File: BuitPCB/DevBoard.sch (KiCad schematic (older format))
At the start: 1 part, among them U1 Teensy4.1

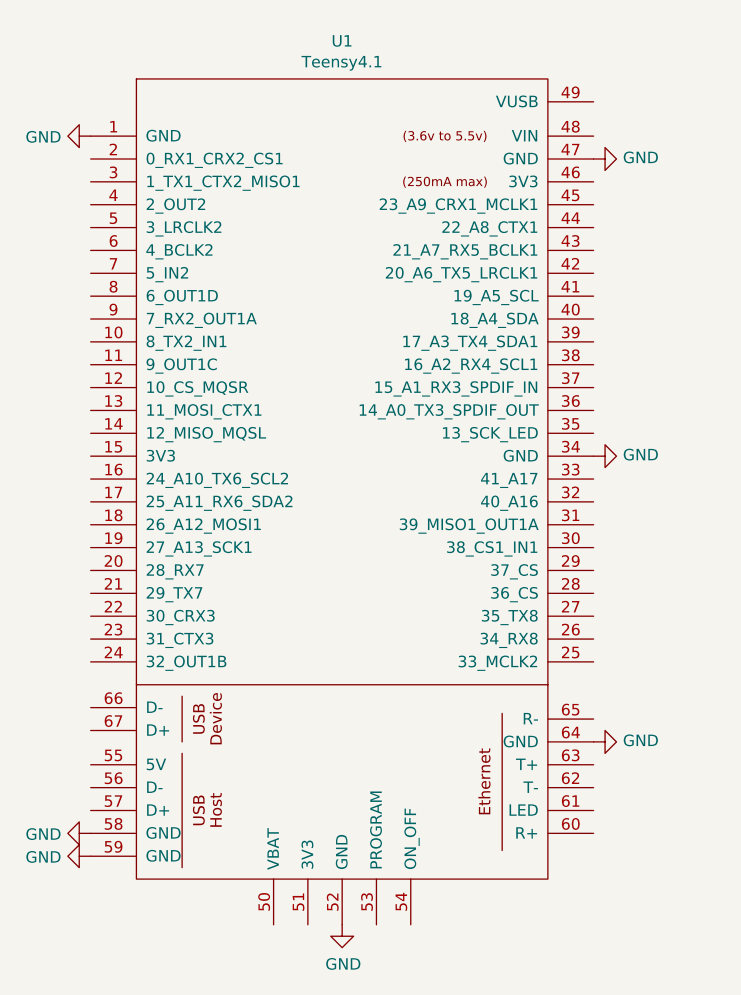
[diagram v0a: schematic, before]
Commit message: Added most of components, few pending
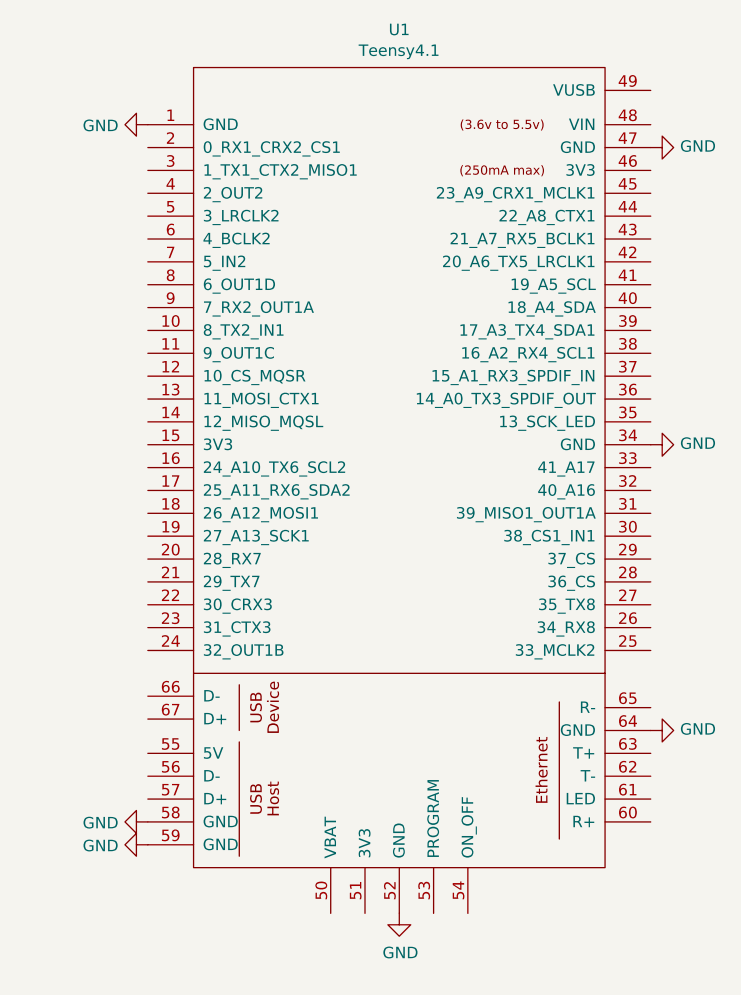
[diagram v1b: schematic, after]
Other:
- moved on the sheet: U1
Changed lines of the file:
@@
 $Descr A4 11693 8268
 encoding utf-8
-Sheet 2 4
+Sheet 2 5
 Title ""
 Date ""
@@
 L teensy:Teensy4.1 U?
 U 1 1 61A96076
-P 5800 4050
+P 6050 4000
 AR Path="/61A96076" Ref="U?"  Part="1"
 AR Path="/61A90B8E/61A96076" Ref="U1"  Part="1"
-F 0 "U1" H 5800 6615 50  0000 C CNN
-F 1 "Teensy4.1" H 5800 6524 50  0000 C CNN
-F 2 "teensy:Teensy41" H 5400 4450 50  0001 C CNN
-F 3 "" H 5400 4450 50  0001 C CNN
-	1    5800 4050
+F 0 "U1" H 6050 6565 50  0000 C CNN
+F 1 "Teensy4.1" H 6050 6474 50  0000 C CNN
+F 2 "teensy:Teensy41" H 5650 4400 50  0001 C CNN
+F 3 "" H 5650 4400 50  0001 C CNN
+	1    6050 4000
 	1    0    0    -1
 $EndComp
@@
 L power:GND #PWR0101
 U 1 1 61A9C991
-P 4700 1900
-F 0 "#PWR0101" H 4700 1650 50  0001 C CNN
-F 1 "GND" V 4705 1772 50  0000 R CNN
-F 2 "" H 4700 1900 50  0001 C CNN
-F 3 "" H 4700 1900 50  0001 C CNN
-	1    4700 1900
+P 4950 1850
+F 0 "#PWR0101" H 4950 1600 50  0001 C CNN
+F 1 "GND" V 4955 1722 50  0000 R CNN
+F 2 "" H 4950 1850 50  0001 C CNN
+F 3 "" H 4950 1850 50  0001 C CNN
+	1    4950 1850
 	0    1    1    0
 $EndComp
@@
 L power:GND #PWR0102
 U 1 1 61A9CF3F
-P 5800 5350
-F 0 "#PWR0102" H 5800 5100 50  0001 C CNN
-F 1 "GND" H 5805 5177 50  0000 C CNN
-F 2 "" H 5800 5350 50  0001 C CNN
-F 3 "" H 5800 5350 50  0001 C CNN
-	1    5800 5350
+P 6050 5300
+F 0 "#PWR0102" H 6050 5050 50  0001 C CNN
+F 1 "GND" H 6055 5127 50  0000 C CNN
+F 2 "" H 6050 5300 50  0001 C CNN
+F 3 "" H 6050 5300 50  0001 C CNN
+	1    6050 5300
 	1    0    0    -1
 $EndComp
@@
 L power:GND #PWR0103
 U 1 1 61A9EF5C
-P 4700 4950
-F 0 "#PWR0103" H 4700 4700 50  0001 C CNN
-F 1 "GND" V 4705 4822 50  0000 R CNN
-F 2 "" H 4700 4950 50  0001 C CNN
-F 3 "" H 4700 4950 50  0001 C CNN
-	1    4700 4950
+P 4950 4900
+F 0 "#PWR0103" H 4950 4650 50  0001 C CNN
+F 1 "GND" V 4955 4772 50  0000 R CNN
+F 2 "" H 4950 4900 50  0001 C CNN
+F 3 "" H 4950 4900 50  0001 C CNN
+	1    4950 4900
 	0    1    1    0
 $EndComp
@@
 L power:GND #PWR0104
 U 1 1 61A9F9EA
-P 4700 5050
-F 0 "#PWR0104" H 4700 4800 50  0001 C CNN
-F 1 "GND" V 4705 4922 50  0000 R CNN
-F 2 "" H 4700 5050 50  0001 C CNN
-F 3 "" H 4700 5050 50  0001 C CNN
-	1    4700 5050
+P 4950 5000
+F 0 "#PWR0104" H 4950 4750 50  0001 C CNN
+F 1 "GND" V 4955 4872 50  0000 R CNN
+F 2 "" H 4950 5000 50  0001 C CNN
+F 3 "" H 4950 5000 50  0001 C CNN
+	1    4950 5000
 	0    1    1    0
 $EndComp
@@
 L power:GND #PWR0105
 U 1 1 61A9FFE0
-P 6900 3300
-F 0 "#PWR0105" H 6900 3050 50  0001 C CNN
-F 1 "GND" V 6905 3172 50  0000 R CNN
-F 2 "" H 6900 3300 50  0001 C CNN
-F 3 "" H 6900 3300 50  0001 C CNN
-	1    6900 3300
+P 7150 3250
+F 0 "#PWR0105" H 7150 3000 50  0001 C CNN
+F 1 "GND" V 7155 3122 50  0000 R CNN
+F 2 "" H 7150 3250 50  0001 C CNN
+F 3 "" H 7150 3250 50  0001 C CNN
+	1    7150 3250
 	0    -1   -1   0
 $EndComp
@@
 L power:GND #PWR0106
 U 1 1 61AA08C4
-P 6900 2000
-F 0 "#PWR0106" H 6900 1750 50  0001 C CNN
-F 1 "GND" V 6905 1872 50  0000 R CNN
-F 2 "" H 6900 2000 50  0001 C CNN
-F 3 "" H 6900 2000 50  0001 C CNN
-	1    6900 2000
+P 7150 1950
+F 0 "#PWR0106" H 7150 1700 50  0001 C CNN
+F 1 "GND" V 7155 1822 50  0000 R CNN
+F 2 "" H 7150 1950 50  0001 C CNN
+F 3 "" H 7150 1950 50  0001 C CNN
+	1    7150 1950
 	0    -1   -1   0
 $EndComp
@@
 L power:GND #PWR0107
 U 1 1 61AA1181
-P 6900 4550
-F 0 "#PWR0107" H 6900 4300 50  0001 C CNN
-F 1 "GND" V 6905 4422 50  0000 R CNN
-F 2 "" H 6900 4550 50  0001 C CNN
-F 3 "" H 6900 4550 50  0001 C CNN
-	1    6900 4550
+P 7150 4500
+F 0 "#PWR0107" H 7150 4250 50  0001 C CNN
+F 1 "GND" V 7155 4372 50  0000 R CNN
+F 2 "" H 7150 4500 50  0001 C CNN
+F 3 "" H 7150 4500 50  0001 C CNN
+	1    7150 4500
 	0    -1   -1   0
 $EndComp
